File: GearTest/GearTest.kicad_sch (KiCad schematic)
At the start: 25 parts, among them J1 Jack-DC, J2 Терминал выключателя моторов, J3 Терминал выключателя основног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, J4 Терминалы XY-FZ35, J5 Терминал питания XY-FZ35, J6 Терминал LCD_1602_I2C, J7 Терминал UART1, M1 Motor_DC, M2 Motor_DC, Q1 IRLZ44N, SW1 Выключатель моторов, SW2 Выключатель основного питания, SW3 SW_Push, U1 WeAct BlackPill STM32F411C_C-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, U2 CH340N, U3 INA219

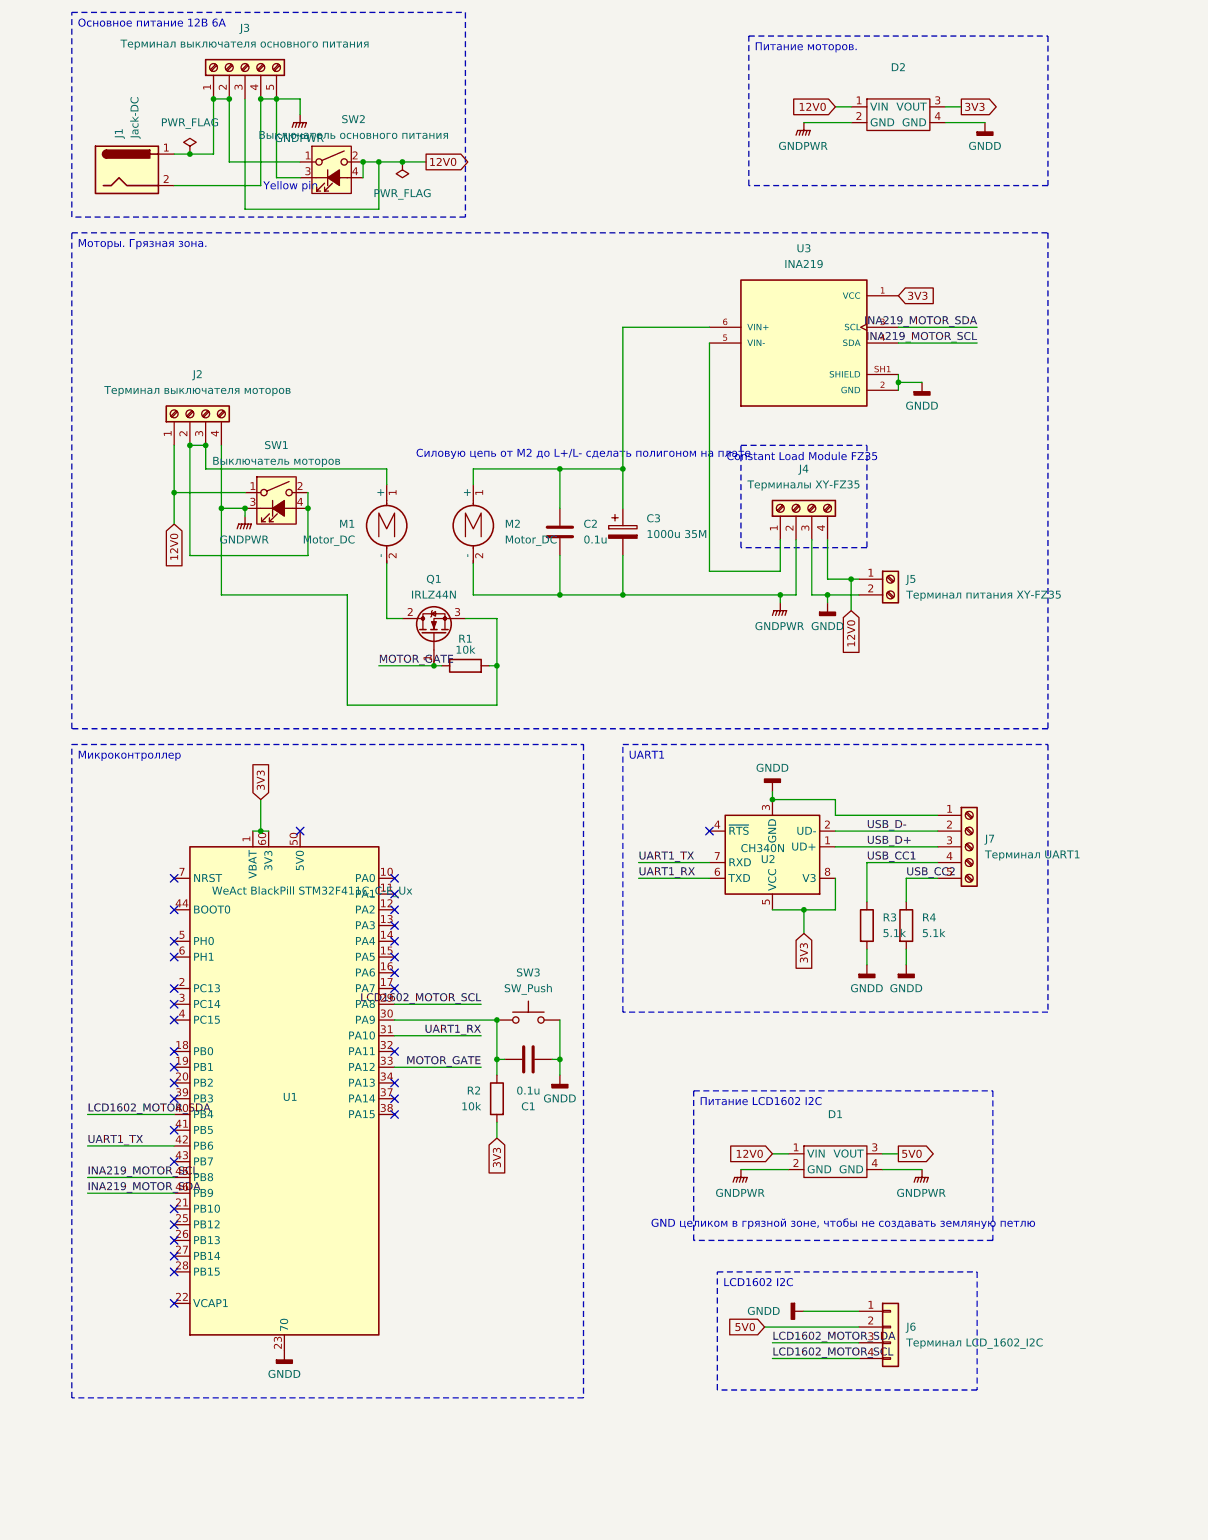
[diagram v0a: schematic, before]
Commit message: dev
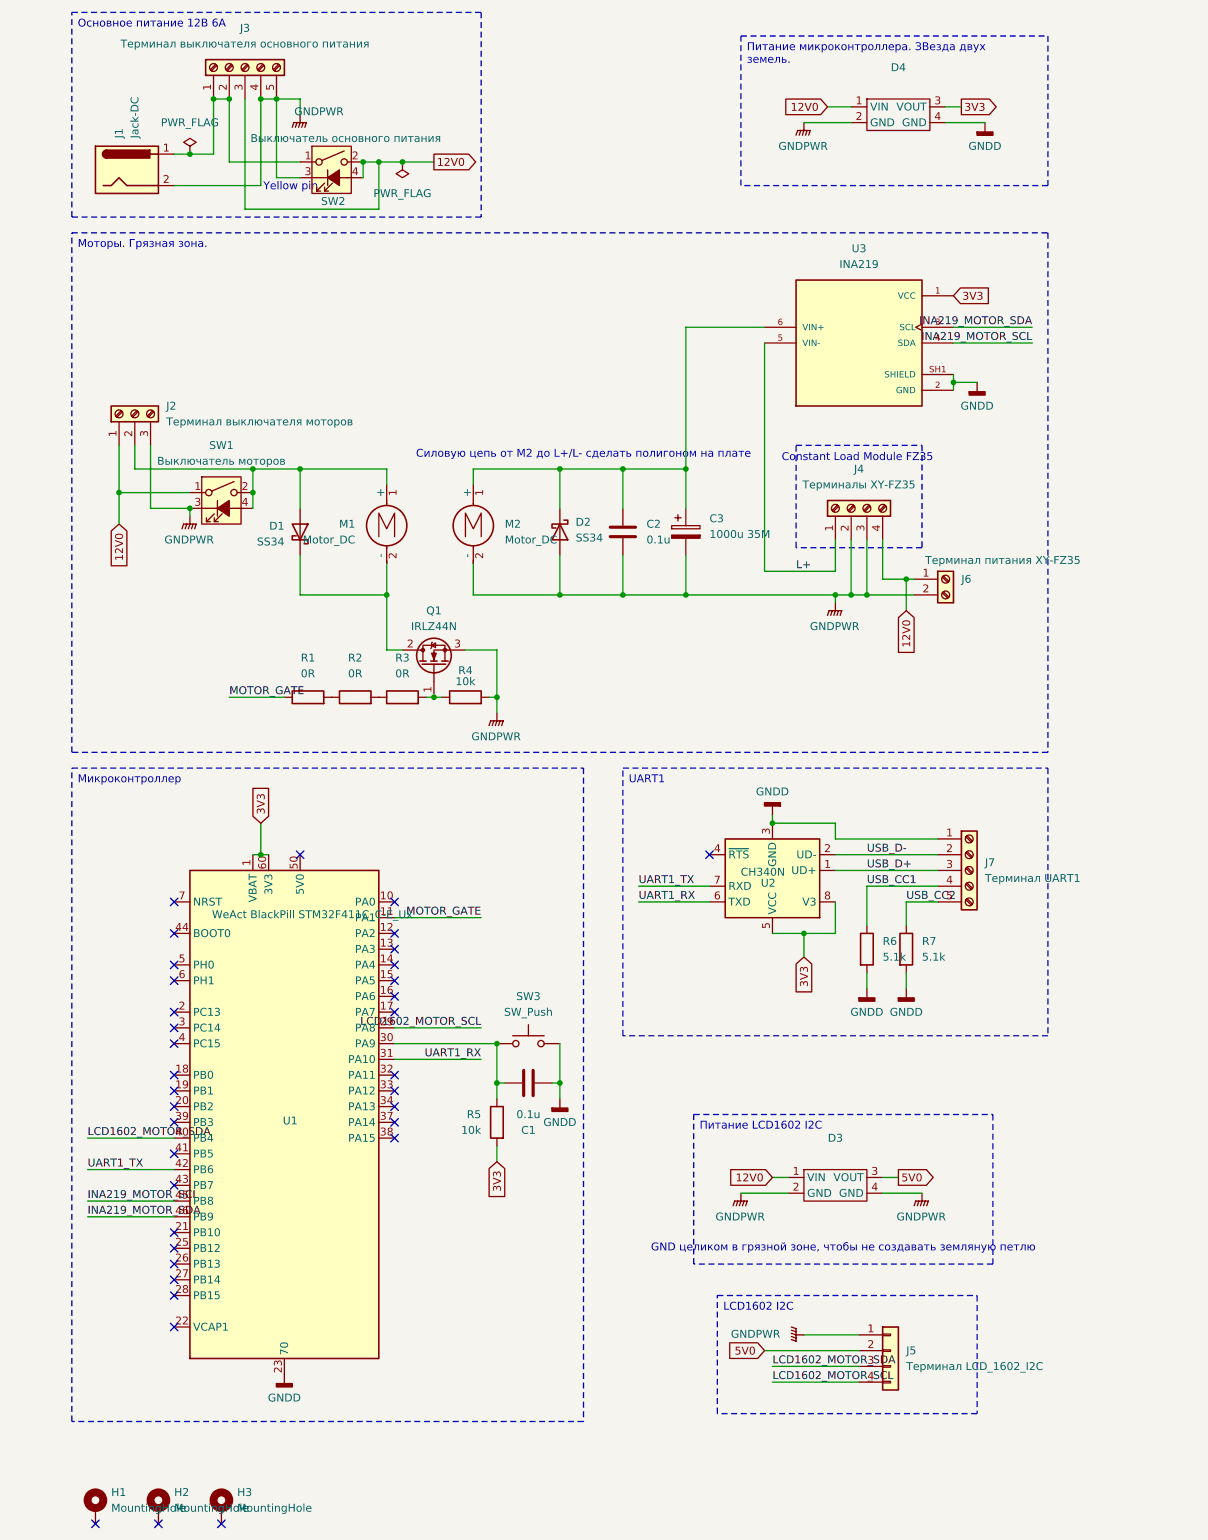
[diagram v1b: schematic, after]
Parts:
- added D1, D2: SS34, Diode_SMD:D_SMA, symbol Diode:SS34
- added H1, H2, H3: MountingHole, MountingHole:MountingHole_2.2mm_M2_DIN965_Pad_TopOnly, symbol Mechanical:MountingHole_Pad
- added R1, R2, R3: 0R, Resistor_SMD:R_2512_6332Metric_Pad1.40x3.35mm_HandSolder, symbol Device:R
- J2: footprint TerminalBlock_Phoenix:TerminalBlock_Phoenix_MPT-0,5-5-2.54_1x05_P2.54mm_Horizontal -> TerminalBlock_Phoenix:TerminalBlock_Phoenix_MPT-0,5-3-2.54_1x03_P2.54mm_Horizontal; symbol Connector:Screw_Terminal_01x04 -> Connector:Screw_Terminal_01x03
- R4: renamed from R1; footprint (none) -> Resistor_SMD:R_0603_1608Metric_Pad0.98x0.95mm_HandSolder
- renumbered D1 to D3, D2 to D4, J6 to J5, J5 to J6, R2 to R5, R3 to R6, R4 to R7
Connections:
- net GNDD: no longer J4.3 (Pin_3), J5.1 (Pin_1), J6.2 (Pin_2)
- net GNDPWR: now also J2.3 (Pin_3), J4.3 (Pin_3), J5.1 (Pin_1), J6.2 (Pin_2), D2.2 (A); no longer J2.4 (Pin_4)
- net MOTOR_GATE: now also U1.11 (PA1), R1.1; no longer Q1.1 (G), R4.1, U1.33 (PA12)
- net at J2.2 (Pin_2), M1.1 (+), SW1.2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: now also D1.2 (A); no longer J2.3 (Pin_3)
- net at C2.1, C3.1, M2.1 (+)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: now also D2.1 (K)
- net at M1.2 (-), Q1.2 (D): now also D1.1 (K)
- net L+: now reaches J4.1 (Pin_1), U3.5 (VIN-), U3.VIN-
- new net: R1.2, R2.1
- new net: R2.2, R3.1
- new net: Q1.1 (G), R3.2, R4.1
- no-connect marks 33 -> 36
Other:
- moved on the sheet: C1, C2, C3, D3, J4, J5, J6, J7, Q1, R4, R5, R6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
